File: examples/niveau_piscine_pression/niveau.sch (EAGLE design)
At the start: 10 parts, among them IC1 MCP6241-E_P, IC2 L7805ACV, IC3 MCP3201-CI_P, J1 DCJ0202, U1 MPX2010DP, U2 D1_MINI

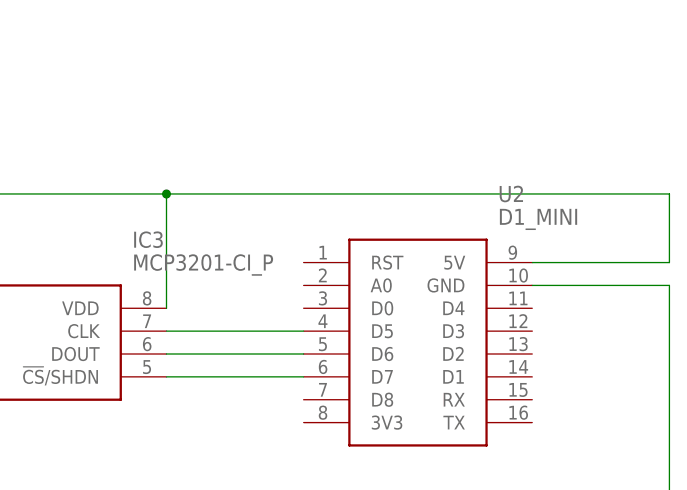
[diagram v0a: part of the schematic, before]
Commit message: Piscine : niveau
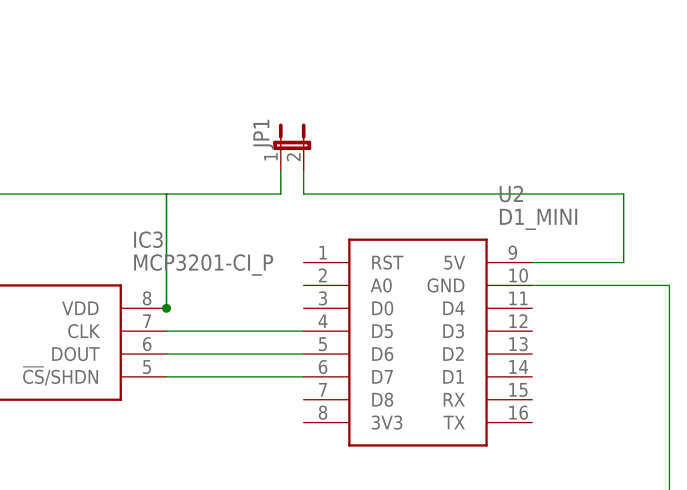
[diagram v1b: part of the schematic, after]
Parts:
- added JP1: (no value), jumper:JP1E
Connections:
- new net N$8: JP1.2, U2.5V
- net N$6: now also JP1.1; no longer U2.5V
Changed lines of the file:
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@@
 <part name="IC3" library="MCP3201-CI_P" deviceset="MCP3201-CI_P" device=""/>
 <part name="U2" library="D1_Mini" deviceset="D1_MINI" device=""/>
+<part name="JP1" library="jumper" library_urn="urn:adsk.eagle:library:252" deviceset="JP1E" device="" package3d_urn="urn:adsk.eagle:package:15455/1"/>
 </parts>
 <sheets>
@@
 <instance part="IC3" gate="G$1" x="129.54" y="71.12"/>
 <instance part="U2" gate="G$1" x="180.34" y="76.2"/>
+<instance part="JP1" gate="A" x="177.8" y="88.9"/>
 </instances>
 <busses>
@@
 <wire x1="129.54" y1="83.82" x2="129.54" y2="71.12" width="0.1524" layer="91"/>
 <junction x="129.54" y="71.12"/>
-<junction x="165.1" y="83.82"/>
-<pinref part="U2" gate="G$1" pin="5V"/>
-<wire x1="220.98" y1="83.82" x2="165.1" y2="83.82" width="0.1524" layer="91"/>
-<wire x1="205.74" y1="76.2" x2="220.98" y2="76.2" width="0.1524" layer="91"/>
-<wire x1="220.98" y1="76.2" x2="220.98" y2="83.82" width="0.1524" layer="91"/>
+<wire x1="165.1" y1="71.12" x2="165.1" y2="83.82" width="0.1524" layer="91"/>
+<wire x1="165.1" y1="83.82" x2="177.8" y2="83.82" width="0.1524" layer="91"/>
+<junction x="165.1" y="71.12"/>
+<pinref part="JP1" gate="A" pin="1"/>
+<wire x1="177.8" y1="83.82" x2="177.8" y2="86.36" width="0.1524" layer="91"/>
 </segment>
 </net>
@@
 </segment>
 </net>
+<net name="N$8" class="0">
+<segment>
+<pinref part="JP1" gate="A" pin="2"/>
+<wire x1="180.34" y1="86.36" x2="180.34" y2="83.82" width="0.1524" layer="91"/>
+<wire x1="180.34" y1="83.82" x2="215.9" y2="83.82" width="0.1524" layer="91"/>
+<wire x1="215.9" y1="83.82" x2="215.9" y2="76.2" width="0.1524" layer="91"/>
+<pinref part="U2" gate="G$1" pin="5V"/>
+<wire x1="215.9" y1="76.2" x2="205.74" y2="76.2" width="0.1524" layer="91"/>
+</segment>
+</net>

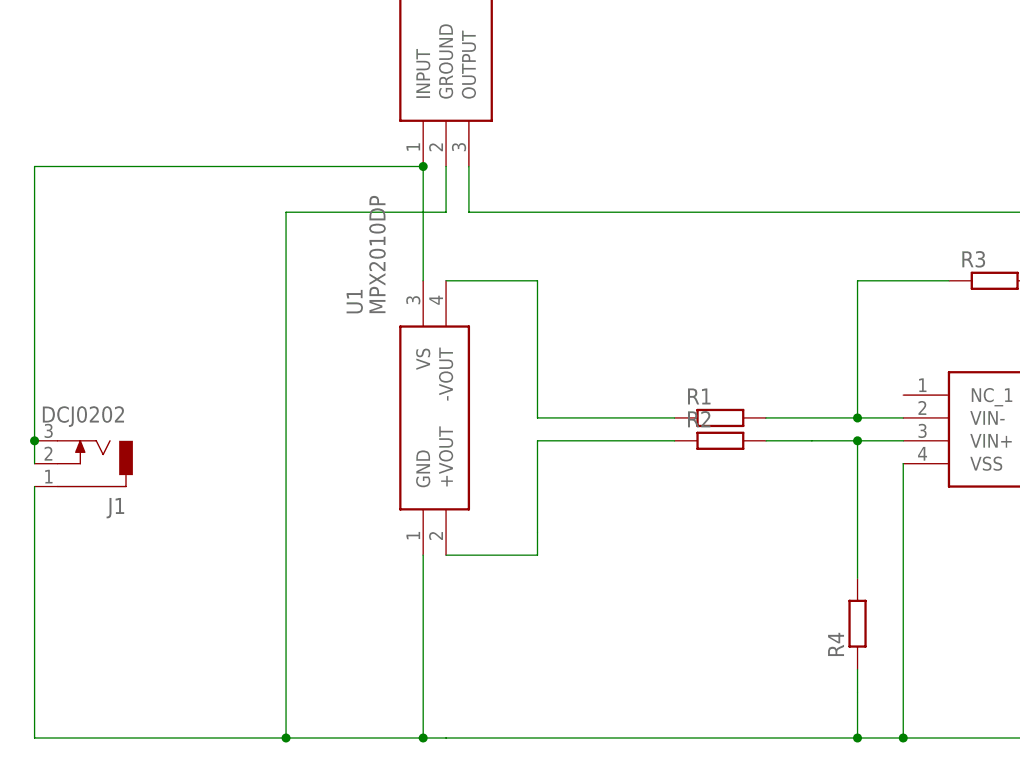
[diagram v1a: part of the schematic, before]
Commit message: Add files via upload
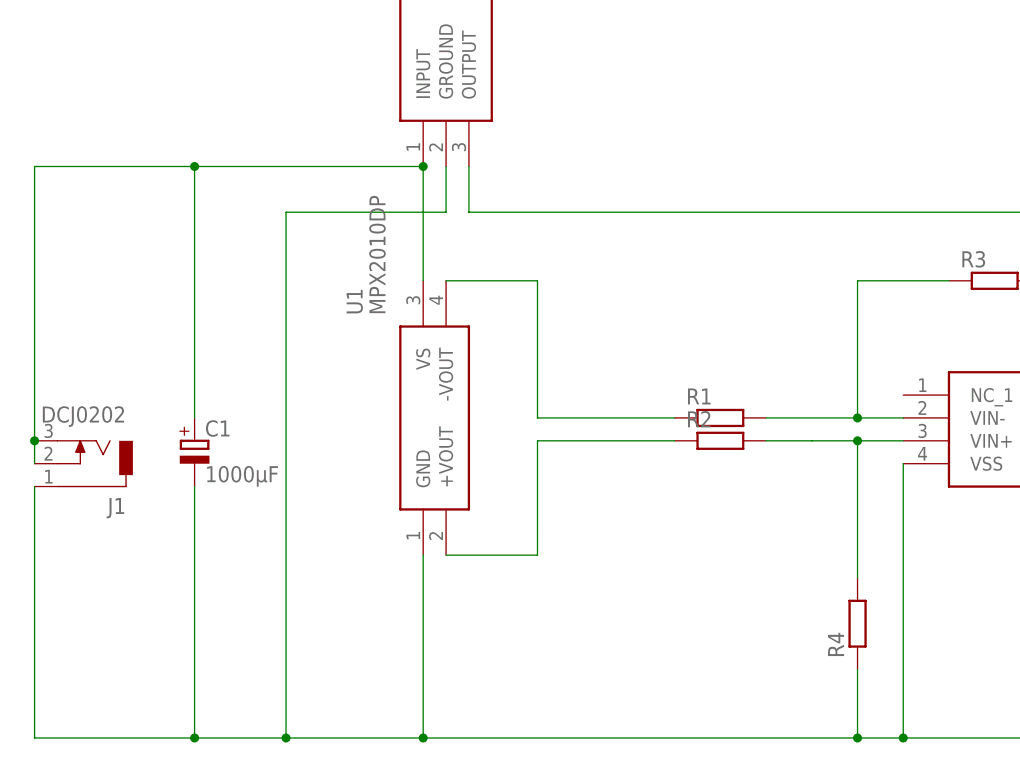
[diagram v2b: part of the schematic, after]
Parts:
- added C1: 1000µF, rcl:CPOL-EUE10-35
- R1, R2, R3, R4: device resistor:R-EU_0204/2V -> rcl:R-EU_0309/10
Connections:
- net N$3: now also C1.-
- net N$4: now also C1.+
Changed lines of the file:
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@@
 <?xml version="1.0" encoding="utf-8"?>
 <!DOCTYPE eagle SYSTEM "eagle.dtd">
-<eagle version="9.1.0">
+<eagle version="8.5.2">
 <drawing>
 <settings>
@@
 <part name="IC2" library="L7805ACV" deviceset="L7805ACV" device=""/>
 <part name="U1" library="MPX2010DP" deviceset="MPX2010DP" device=""/>
-<part name="R1" library="resistor" library_urn="urn:adsk.eagle:library:348" deviceset="R-EU_" device="0204/2V" package3d_urn="urn:adsk.eagle:package:25948/1"/>
-<part name="R2" library="resistor" library_urn="urn:adsk.eagle:library:348" deviceset="R-EU_" device="0204/2V" package3d_urn="urn:adsk.eagle:package:25948/1"/>
-<part name="R3" library="resistor" library_urn="urn:adsk.eagle:library:348" deviceset="R-EU_" device="0204/2V" package3d_urn="urn:adsk.eagle:package:25948/1"/>
-<part name="R4" library="resistor" library_urn="urn:adsk.eagle:library:348" deviceset="R-EU_" device="0204/2V" package3d_urn="urn:adsk.eagle:package:25948/1"/>
+<part name="R1" library="rcl" library_urn="urn:adsk.eagle:library:334" deviceset="R-EU_" device="0309/10" package3d_urn="urn:adsk.eagle:package:23567/1"/>
+<part name="R2" library="rcl" library_urn="urn:adsk.eagle:library:334" deviceset="R-EU_" device="0309/10" package3d_urn="urn:adsk.eagle:package:23567/1"/>
+<part name="R3" library="rcl" library_urn="urn:adsk.eagle:library:334" deviceset="R-EU_" device="0309/10" package3d_urn="urn:adsk.eagle:package:23567/1"/>
+<part name="R4" library="rcl" library_urn="urn:adsk.eagle:library:334" deviceset="R-EU_" device="0309/10" package3d_urn="urn:adsk.eagle:package:23567/1"/>
 <part name="J1" library="con-jack" library_urn="urn:adsk.eagle:library:154" deviceset="DCJ0202" device="" package3d_urn="urn:adsk.eagle:package:7491/1"/>
 <part name="IC3" library="MCP3201-CI_P" deviceset="MCP3201-CI_P" device=""/>
 <part name="U2" library="D1_Mini" deviceset="D1_MINI" device=""/>
 <part name="JP1" library="jumper" library_urn="urn:adsk.eagle:library:252" deviceset="JP1E" device="" package3d_urn="urn:adsk.eagle:package:15455/1"/>
+<part name="C1" library="rcl" library_urn="urn:adsk.eagle:library:334" deviceset="CPOL-EU" device="E10-35" package3d_urn="urn:adsk.eagle:package:23395/1" value="1000µF"/>
 </parts>
 <sheets>
@@
 <instance part="U2" gate="G$1" x="180.34" y="76.2"/>
 <instance part="JP1" gate="A" x="177.8" y="88.9"/>
+<instance part="C1" gate="G$1" x="-25.4" y="45.72"/>
 </instances>
 <busses>
@@
 <pinref part="U1" gate="G$1" pin="GND"/>
 <wire x1="0" y1="33.02" x2="0" y2="12.7" width="0.1524" layer="91"/>
-<wire x1="0" y1="12.7" x2="2.54" y2="12.7" width="0.1524" layer="91"/>
 <pinref part="IC1" gate="G$1" pin="VSS"/>
-<wire x1="2.54" y1="12.7" x2="48.26" y2="12.7" width="0.1524" layer="91"/>
+<wire x1="0" y1="12.7" x2="48.26" y2="12.7" width="0.1524" layer="91"/>
 <wire x1="48.26" y1="12.7" x2="53.34" y2="12.7" width="0.1524" layer="91"/>
 <wire x1="53.34" y1="12.7" x2="53.34" y2="43.18" width="0.1524" layer="91"/>
@@
 <junction x="0" y="12.7"/>
 <pinref part="R4" gate="G$1" pin="1"/>
-<wire x1="48.26" y1="20.32" x2="48.26" y2="17.78" width="0.1524" layer="91"/>
-<wire x1="48.26" y1="17.78" x2="48.26" y2="12.7" width="0.1524" layer="91"/>
+<wire x1="48.26" y1="20.32" x2="48.26" y2="12.7" width="0.1524" layer="91"/>
 <junction x="48.26" y="12.7"/>
 <pinref part="J1" gate="G$1" pin="1"/>
 <wire x1="-43.18" y1="40.64" x2="-43.18" y2="12.7" width="0.1524" layer="91"/>
-<wire x1="-43.18" y1="12.7" x2="-15.24" y2="12.7" width="0.1524" layer="91"/>
+<wire x1="-43.18" y1="12.7" x2="-25.4" y2="12.7" width="0.1524" layer="91"/>
 <junction x="-15.24" y="12.7"/>
 <pinref part="IC3" gate="G$1" pin="VSS"/>
+<wire x1="-25.4" y1="12.7" x2="-15.24" y2="12.7" width="0.1524" layer="91"/>
 <wire x1="129.54" y1="63.5" x2="129.54" y2="12.7" width="0.1524" layer="91"/>
 <wire x1="129.54" y1="12.7" x2="53.34" y2="12.7" width="0.1524" layer="91"/>
@@
 <wire x1="220.98" y1="12.7" x2="129.54" y2="12.7" width="0.1524" layer="91"/>
 <junction x="129.54" y="12.7"/>
+<pinref part="C1" gate="G$1" pin="-"/>
+<wire x1="-25.4" y1="40.64" x2="-25.4" y2="12.7" width="0.1524" layer="91"/>
+<junction x="-25.4" y="12.7"/>
 </segment>
 </net>
@@
 <wire x1="-43.18" y1="43.18" x2="-43.18" y2="45.72" width="0.1524" layer="91"/>
 <wire x1="-43.18" y1="45.72" x2="-43.18" y2="76.2" width="0.1524" layer="91"/>
-<wire x1="-43.18" y1="76.2" x2="0" y2="76.2" width="0.1524" layer="91"/>
+<wire x1="-43.18" y1="76.2" x2="-25.4" y2="76.2" width="0.1524" layer="91"/>
 <junction x="0" y="76.2"/>
 <pinref part="J1" gate="G$1" pin="3"/>
 <junction x="-43.18" y="45.72"/>
+<pinref part="C1" gate="G$1" pin="+"/>
+<wire x1="-25.4" y1="76.2" x2="0" y2="76.2" width="0.1524" layer="91"/>
+<wire x1="-25.4" y1="48.26" x2="-25.4" y2="76.2" width="0.1524" layer="91"/>
+<junction x="-25.4" y="76.2"/>
 </segment>
 </net>
@@
 packages will not be understood (or retained) with this version.
 </note>
+<note version="8.4" severity="warning">
+Since Version 8.4, EAGLE supports properties for SPICE simulation.
+Probes in schematics and SPICE mapping objects found in parts and library devices
+will not be understood with this version. Update EAGLE to the latest version
+for full support of SPICE simulation.
+</note>
 </compatibility>
